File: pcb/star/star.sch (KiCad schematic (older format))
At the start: 34 parts, among them J1 POWER, J2 program, SW1 RST, SW2 PRG, U1 ESP-12F, U2 AP2112K-3.3

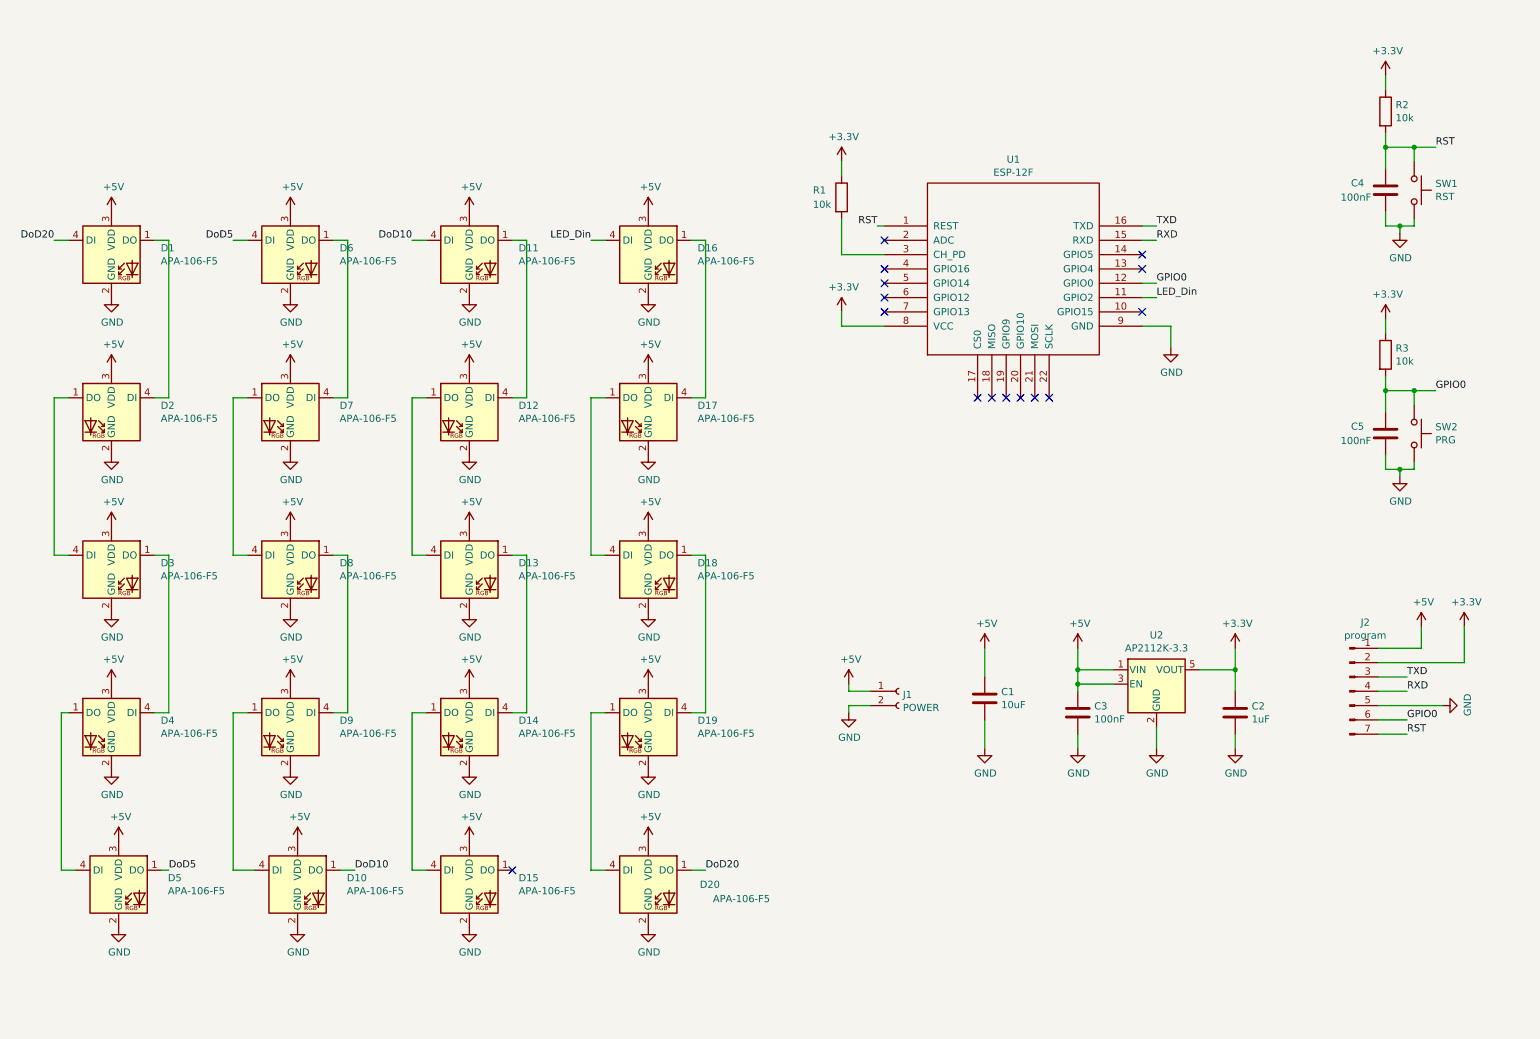
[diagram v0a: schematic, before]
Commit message: ibom added
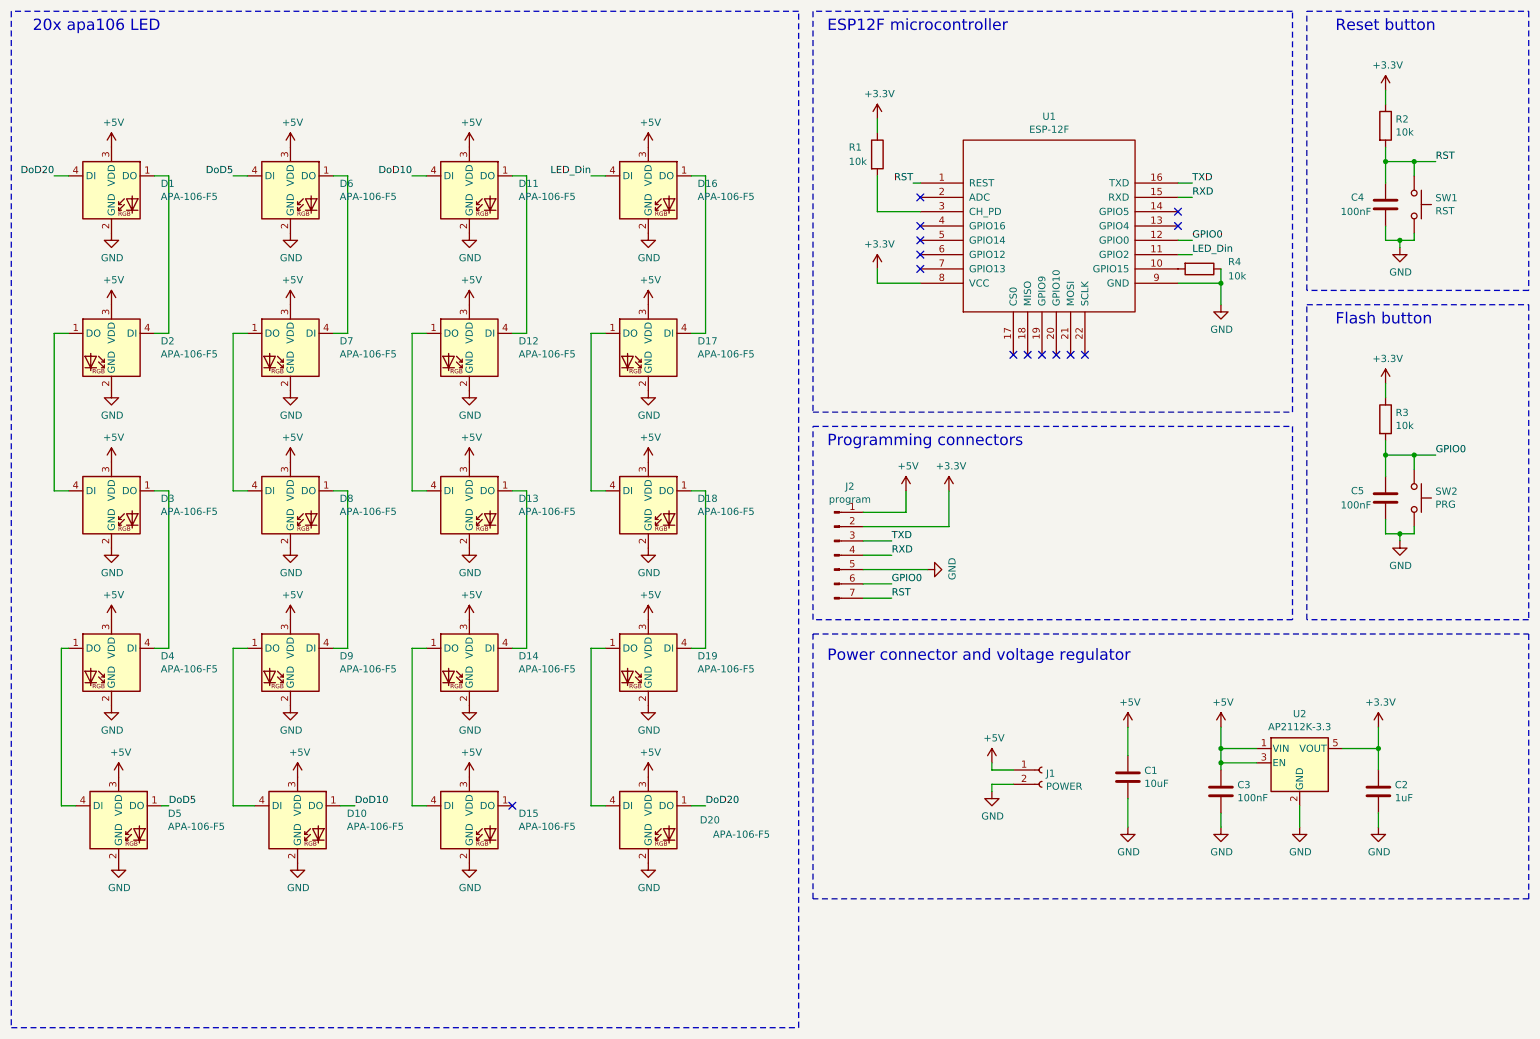
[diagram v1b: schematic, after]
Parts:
- added R4: 10k, Resistor_THT:R_Axial_DIN0204_L3.6mm_D1.6mm_P7.62mm_Horizontal, symbol Device:R
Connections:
- net GND: now also R4.1
- net at U1.10 (GPIO15): now also R4.2
- no-connect marks 15 -> 14
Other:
- note added: "20x apa106 LED"
- note added: "ESP12F microcontroller"
- note added: "Flash button"
- note added: "Power connector and voltage regulator"
- note added: "Programming connectors\n"
- note added: "Reset button"
- moved on the sheet: C1, C2, C3, C4, C5, D1, D10, D11, D12, D13, D14, D15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
